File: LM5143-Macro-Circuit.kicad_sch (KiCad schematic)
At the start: 52 parts, among them J5 SYNC_OUT, J8 SYNC_IN, U21 LM5145, U22 NTMFS4D0N08XT1G, U23 NTMFS4D0N08XT1G, U24 NTMFS4D0N08XT1G, U25 NTMFS4D0N08XT1G

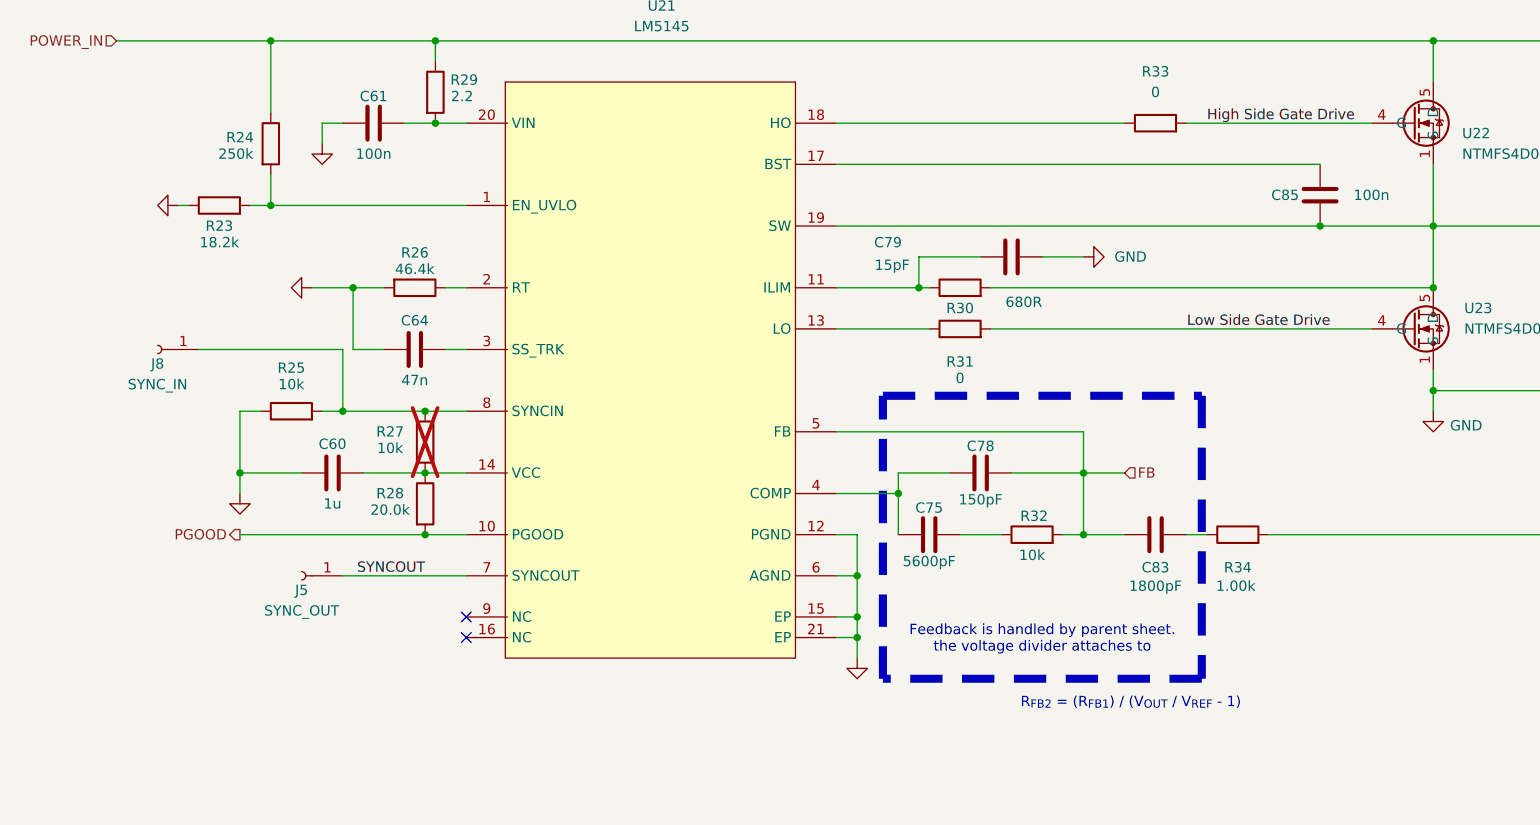
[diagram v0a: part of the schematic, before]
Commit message: Done
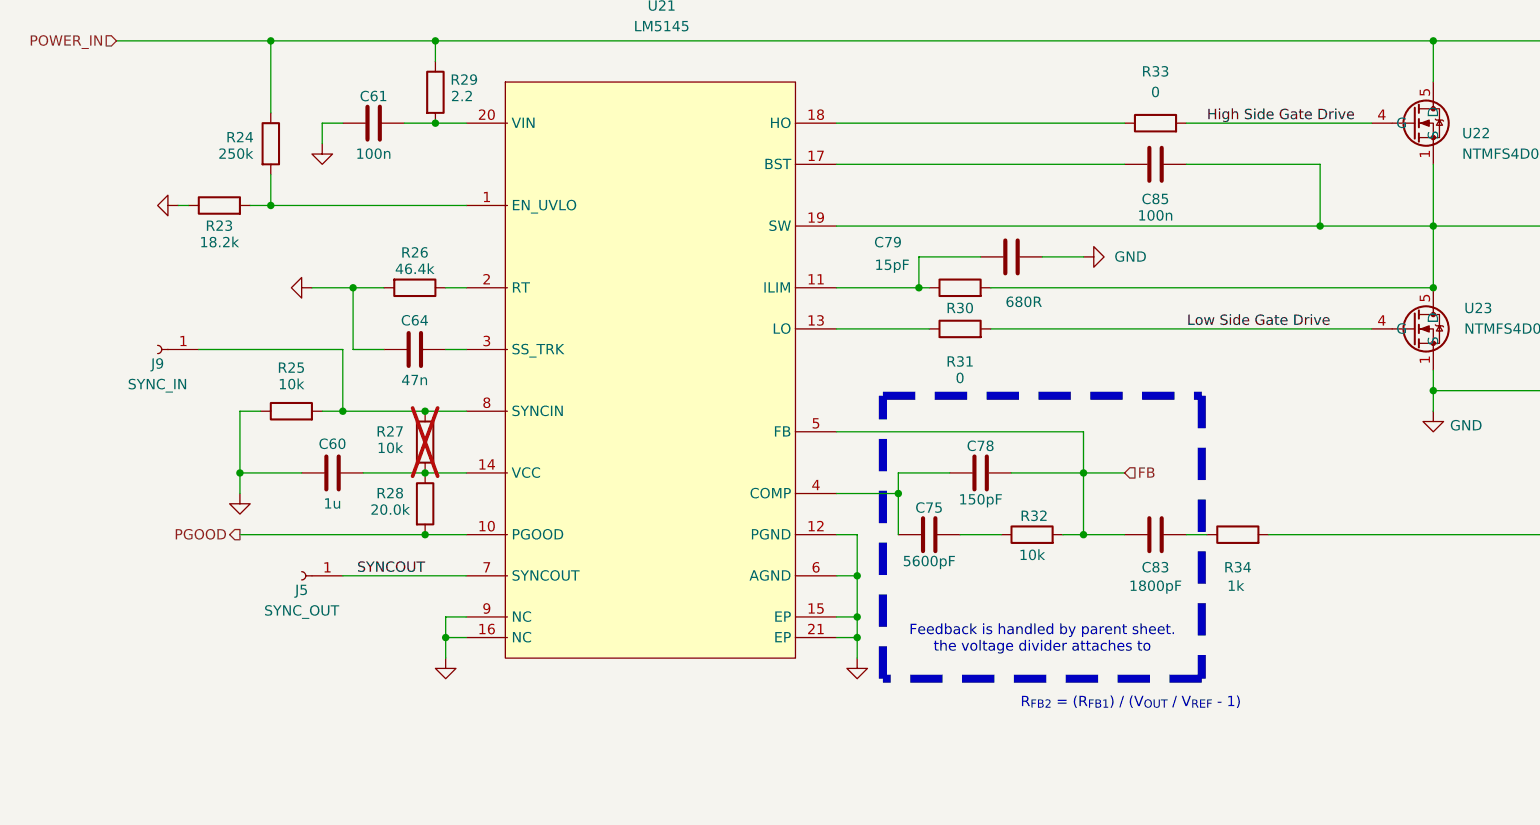
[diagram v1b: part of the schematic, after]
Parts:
- R25, R26, R27, R28, R29, R30, R31, R32, R33: footprint Resistor_SMD:R_0805_2012Metric -> Resistor_SMD:R_0603_1608Metric
- R34: value 1.00k -> 1k; footprint Resistor_SMD:R_0805_2012Metric -> Resistor_SMD:R_0603_1608Metric
- renumbered J8 to J9
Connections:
- net GND: now also U21.16 (NC), U21.9 (NC)
- no-connect marks 2 -> 0
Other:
- moved on the sheet: C85
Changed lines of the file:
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@@
 	)
 	(junction
+		(at 66.04 132.08)
+		(diameter 0)
+		(color 0 0 0 0)
+	)
+	(junction
 		(at 44.45 58.42)
 		(diameter 0)
@@
 		(color 0 0 0 0)
 	)
-	(no_connect
-		(at 68.58 132.08)
-	)
-	(no_connect
-		(at 68.58 129.54)
-	)
 	(wire
 		(pts
@@
 	(wire
 		(pts
-			(xy 114.3 73.66) (xy 173.99 73.66)
+			(xy 114.3 73.66) (xy 149.86 73.66)
+		)
+		(stroke
+			(width 0)
+			(type default)
+		)
+	)
+	(wire
+		(pts
+			(xy 173.99 73.66) (xy 173.99 81.28)
 		)
 		(stroke
@@
 	(wire
 		(pts
+			(xy 66.04 132.08) (xy 68.58 132.08)
+		)
+		(stroke
+			(width 0)
+			(type default)
+		)
+	)
+	(wire
+		(pts
 			(xy 96.52 27.94) (xy 106.68 27.94)
 		)
@@
 	(wire
 		(pts
+			(xy 66.04 134.62) (xy 66.04 132.08)
+		)
+		(stroke
+			(width 0)
+			(type default)
+		)
+	)
+	(wire
+		(pts
 			(xy 130.81 165.1) (xy 130.81 167.64)
 		)
@@
 	(wire
 		(pts
+			(xy 157.48 73.66) (xy 173.99 73.66)
+		)
+		(stroke
+			(width 0)
+			(type default)
+		)
+	)
+	(wire
+		(pts
 			(xy 63.5 119.38) (xy 68.58 119.38)
 		)
@@
 	(wire
 		(pts
+			(xy 66.04 132.08) (xy 66.04 129.54)
+		)
+		(stroke
+			(width 0)
+			(type default)
+		)
+	)
+	(wire
+		(pts
 			(xy 48.26 165.1) (xy 48.26 167.64)
 		)
@@
 	(wire
 		(pts
+			(xy 66.04 129.54) (xy 68.58 129.54)
+		)
+		(stroke
+			(width 0)
+			(type default)
+		)
+	)
+	(wire
+		(pts
 			(xy 48.26 177.8) (xy 48.26 175.26)
 		)
@@
 	(symbol
 		(lib_id "Device:C")
-		(at 173.99 77.47 180)
+		(at 153.67 73.66 270)
 		(unit 1)
 		(exclude_from_sim no)
@@
 		(dnp no)
 		(property "Reference" "C85"
-			(at 169.672 77.47 0)
+			(at 153.67 77.978 90)
 			(effects
 				(font
@@
 		)
 		(property "Value" "100n"
-			(at 180.34 77.47 0)
+			(at 153.67 80.01 90)
 			(effects
 				(font
@@
 		)
 		(property "Footprint" "Capacitor_SMD:C_0603_1608Metric"
-			(at 173.0248 73.66 0)
+			(at 149.86 74.6252 0)
 			(effects
 				(font
@@
 		)
 		(property "Datasheet" "~"
-			(at 173.99 77.47 0)
+			(at 153.67 73.66 0)
 			(effects
 				(font
@@
 		)
 		(property "Description" "Unpolarized capacitor"
-			(at 173.99 77.47 0)
+			(at 153.67 73.66 0)
 			(effects
 				(font
@@
 		(on_board yes)
 		(dnp no)
-		(property "Reference" "J8"
+		(property "Reference" "J9"
 			(at 30.48 98.298 0)
 			(effects
@@
 			)
 		)
-		(property "Footprint" "Resistor_SMD:R_0805_2012Metric"
+		(property "Footprint" "Resistor_SMD:R_0603_1608Metric"
 			(at 61.722 107.95 90)
 			(effects
@@
 	(symbol
 		(lib_id "power:GND")
+		(at 66.04 134.62 0)
+		(unit 1)
+		(exclude_from_sim no)
+		(in_bom yes)
+		(on_board yes)
+		(dnp no)
+		(fields_autoplaced yes)
+		(property "Reference" "#PWR042"
+			(at 66.04 140.97 0)
+			(effects
+				(font
+					(size 1.27 1.27)
+				)
+				(hide yes)
+			)
+		)
+		(property "Value" "GND"
+			(at 66.04 139.7 0)
+			(effects
+				(font
+					(size 1.27 1.27)
+				)
+				(hide yes)
+			)
+		)
+		(property "Footprint" ""
+			(at 66.04 134.62 0)
+			(effects
+				(font
+					(size 1.27 1.27)
+				)
+				(hide yes)
+			)
+		)
+		(property "Datasheet" ""
+			(at 66.04 134.62 0)
+			(effects
+				(font
+					(size 1.27 1.27)
+				)
+				(hide yes)
+			)
+		)
+		(property "Description" "Power symbol creates a global label with name \"GND\" , ground"
+			(at 66.04 134.62 0)
+			(effects
+				(font
+					(size 1.27 1.27)
+				)
+				(hide yes)
+			)
+		)
+		(pin "1"
+		)
+		(instances
+			(project "Battery-Board"
+				(path "/7996c6a7-339e-40c9-8e7c-4c4bf8c43339/0dba19d5-6515-47ba-b397-4a1e13f98b03/18b4f1db-1f57-458d-b3ae-ef62afe7e467"
+					(reference "#PWR093")
+					(unit 1)
+				)
+				(path "/7996c6a7-339e-40c9-8e7c-4c4bf8c43339/0dba19d5-6515-47ba-b397-4a1e13f98b03/d65101b9-3896-47a0-bfde-d52181d0baf1"
+					(reference "#PWR042")
+					(unit 1)
+				)
+			)
+		)
+	)
+	(symbol
+		(lib_id "power:GND")
 		(at 143.51 180.34 0)
 		(unit 1)
@@
 			)
 		)
-		(property "Footprint" "Resistor_SMD:R_0805_2012Metric"
+		(property "Footprint" "Resistor_SMD:R_0603_1608Metric"
 			(at 46.99 105.918 90)
 			(effects
@@
 			)
 		)
-		(property "Footprint" "Resistor_SMD:R_0805_2012Metric"
+		(property "Footprint" "Resistor_SMD:R_0603_1608Metric"
 			(at 129.54 95.758 90)
 			(effects
@@
 			)
 		)
-		(property "Footprint" "Resistor_SMD:R_0805_2012Metric"
+		(property "Footprint" "Resistor_SMD:R_0603_1608Metric"
 			(at 153.67 70.358 90)
 			(effects
@@
 			)
 		)
-		(property "Value" "1.00k"
+		(property "Value" "1k"
 			(at 163.576 125.73 90)
 			(effects
@@
 			)
 		)
-		(property "Footprint" "Resistor_SMD:R_0805_2012Metric"
+		(property "Footprint" "Resistor_SMD:R_0603_1608Metric"
 			(at 163.83 121.158 90)
 			(effects
@@
 			)
 		)
-		(property "Footprint" "Resistor_SMD:R_0805_2012Metric"
+		(property "Footprint" "Resistor_SMD:R_0603_1608Metric"
 			(at 62.23 87.122 90)
 			(effects
@@
 			)
 		)
-		(property "Footprint" "Resistor_SMD:R_0805_2012Metric"
+		(property "Footprint" "Resistor_SMD:R_0603_1608Metric"
 			(at 129.54 90.678 90)
 			(effects
@@
 			)
 		)
-		(property "Footprint" "Resistor_SMD:R_0805_2012Metric"
+		(property "Footprint" "Resistor_SMD:R_0603_1608Metric"
 			(at 138.43 121.158 90)
 			(effects
@@
 			)
 		)
-		(property "Footprint" "Resistor_SMD:R_0805_2012Metric"
+		(property "Footprint" "Resistor_SMD:R_0603_1608Metric"
 			(at 61.722 115.57 90)
 			(effects
@@
 			)
 		)
-		(property "Footprint" "Resistor_SMD:R_0805_2012Metric"
+		(property "Footprint" "Resistor_SMD:R_0603_1608Metric"
 			(at 62.992 64.77 90)
 			(effects
